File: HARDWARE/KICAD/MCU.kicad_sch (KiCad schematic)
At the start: 30 parts, among them U4 STM32F411RET6, Y1 12MHz 18pF, Y2 32.768kHz 12.5pF

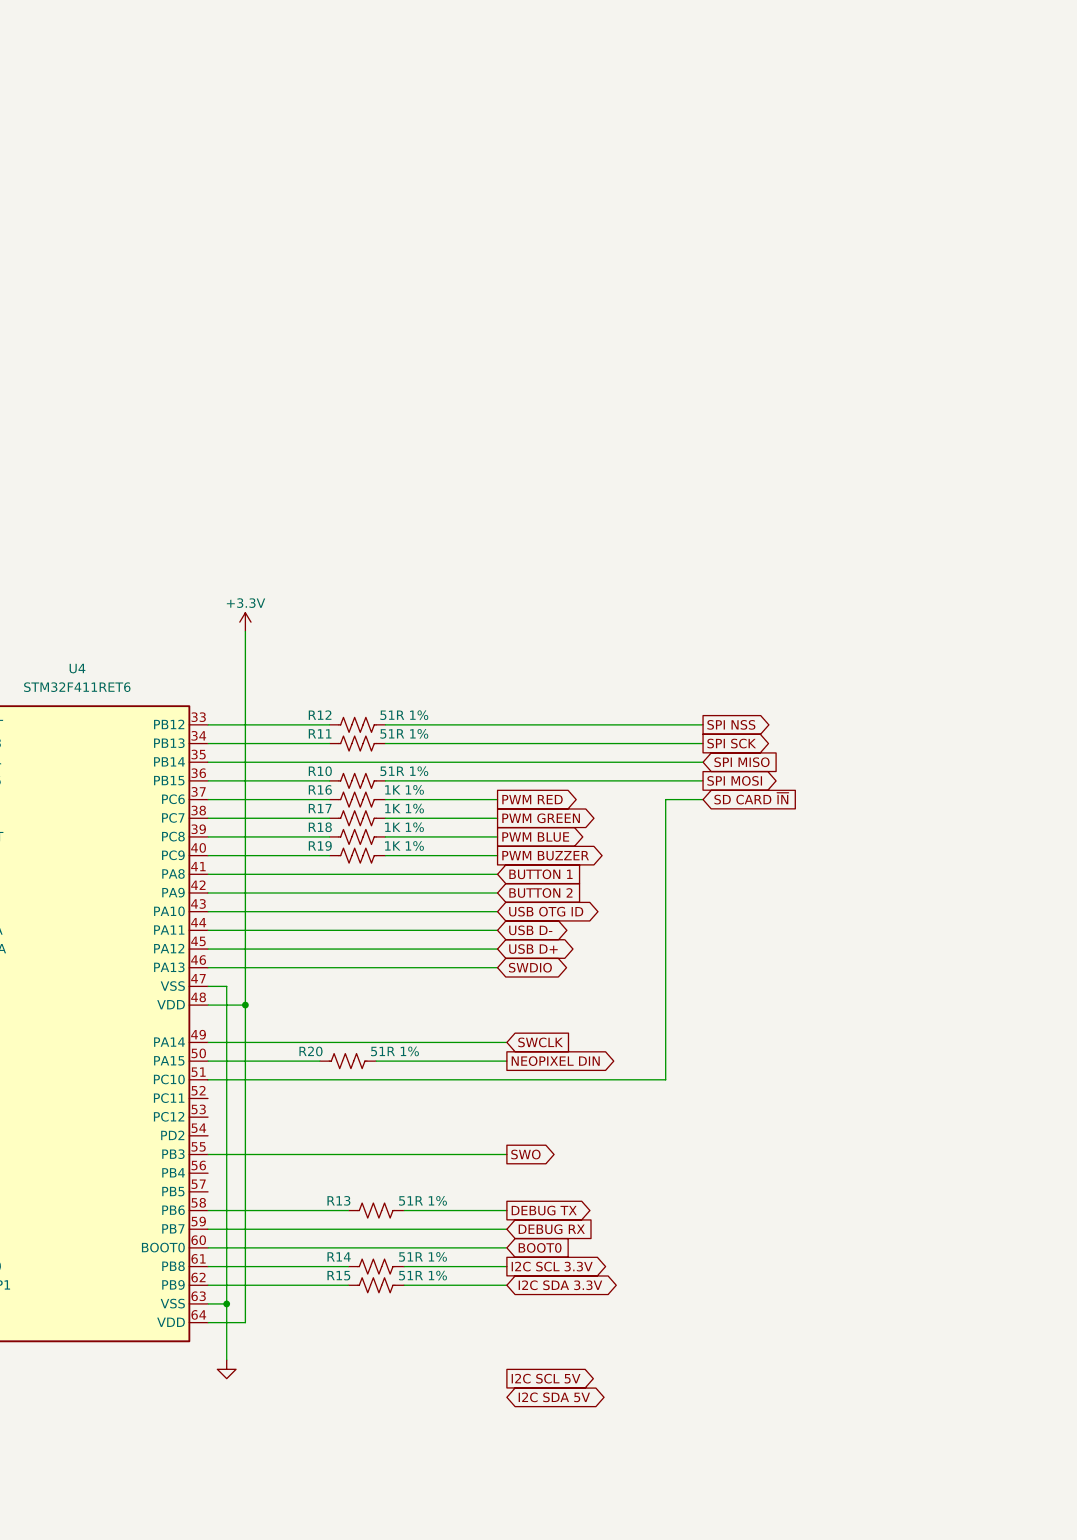
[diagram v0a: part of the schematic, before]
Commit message: Fixed MCU pins on schematic and routed I2C voltage translator.
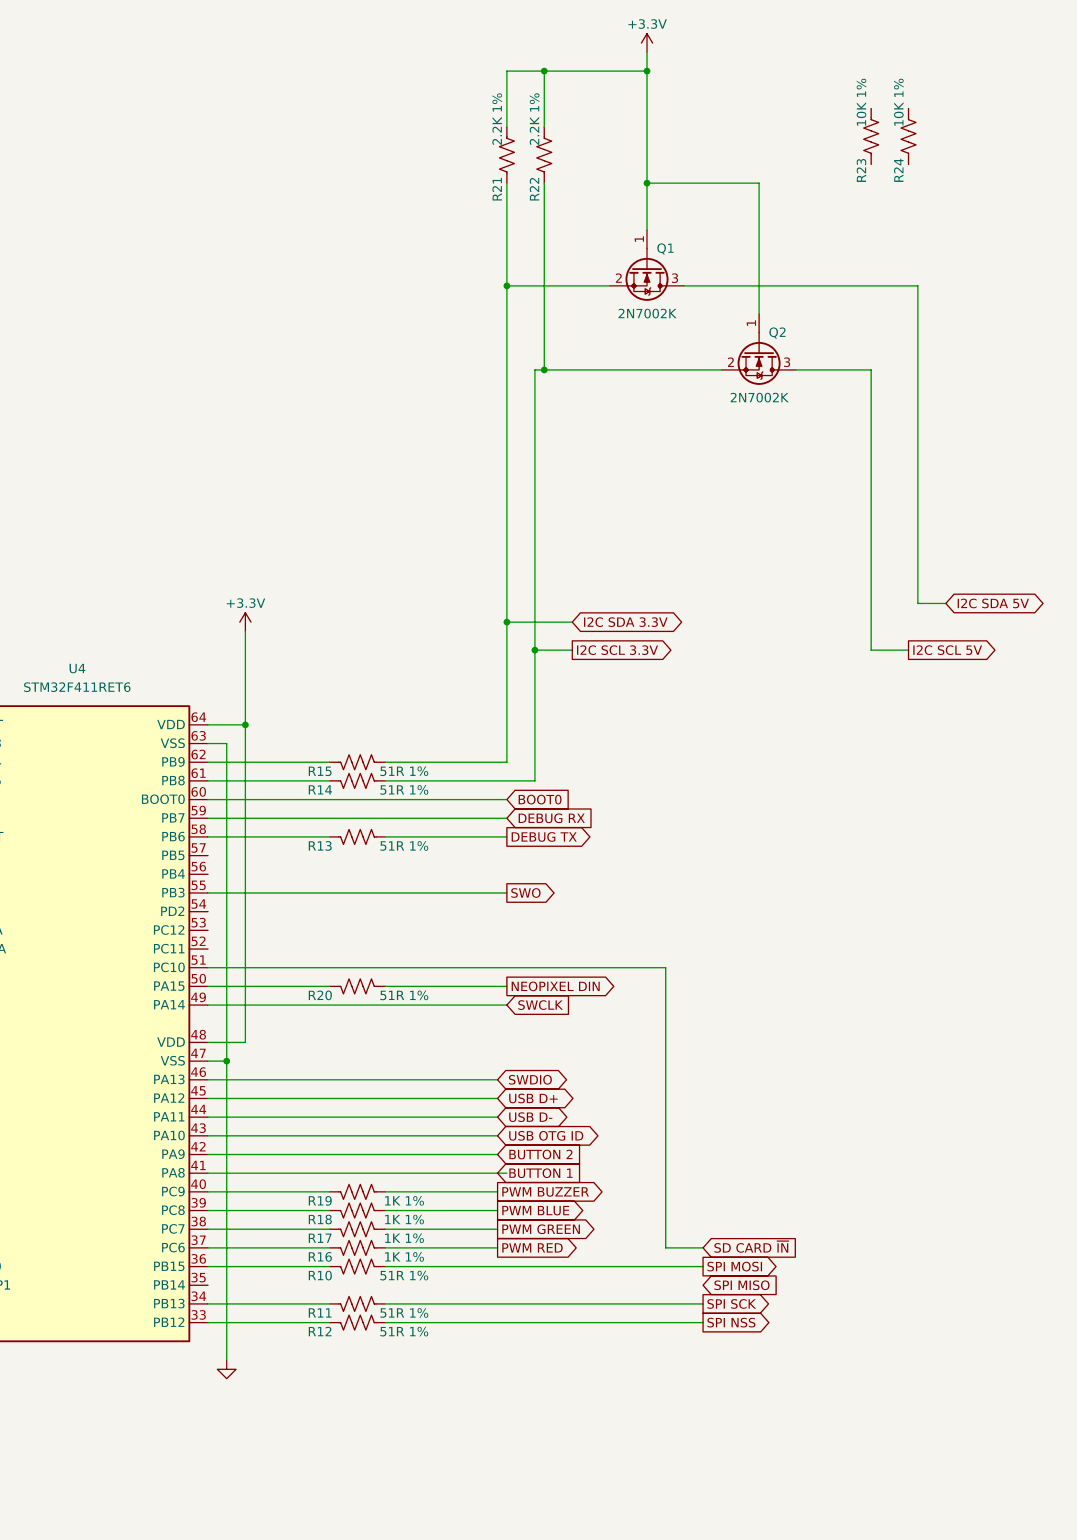
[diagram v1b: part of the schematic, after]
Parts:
- added Q1, Q2: 2N7002K, EMBARCADOS - CURSO PCB:SOT-23, symbol EMBARCADOS - CURSO PCB:TRANSISTOR 2N7002K-7
- added R21, R22: 2.2K 1%, EMBARCADOS - CURSO PCB:R_0603_1608Metric, symbol EMBARCADOS - CURSO PCB:RES 0603 2.2K 1% VISHAY CRCW06032K20FK
- added R23, R24: 10K 1%, EMBARCADOS - CURSO PCB:R_0603_1608Metric, symbol EMBARCADOS - CURSO PCB:RES 0603 10K 1% VISHAY CRCW060310K0FK
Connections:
- net +3.3V: now also Q1.1 (G), Q2.1 (G), R21.1, R22.1
- net I2C SCL 3.3V: now also Q2.2 (S), R22.2
- net I2C SCL 5V: now also Q2.3 (D)
- net I2C SDA 3.3V: now also Q1.2 (S), R21.2
- net I2C SDA 5V: now also Q1.3 (D)
- net SPI MISO: no longer U4.35 (PB14)
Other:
- moved on the sheet: R10, R11, R12, R13, R14, R15, R16, R17, R18, R19, R20

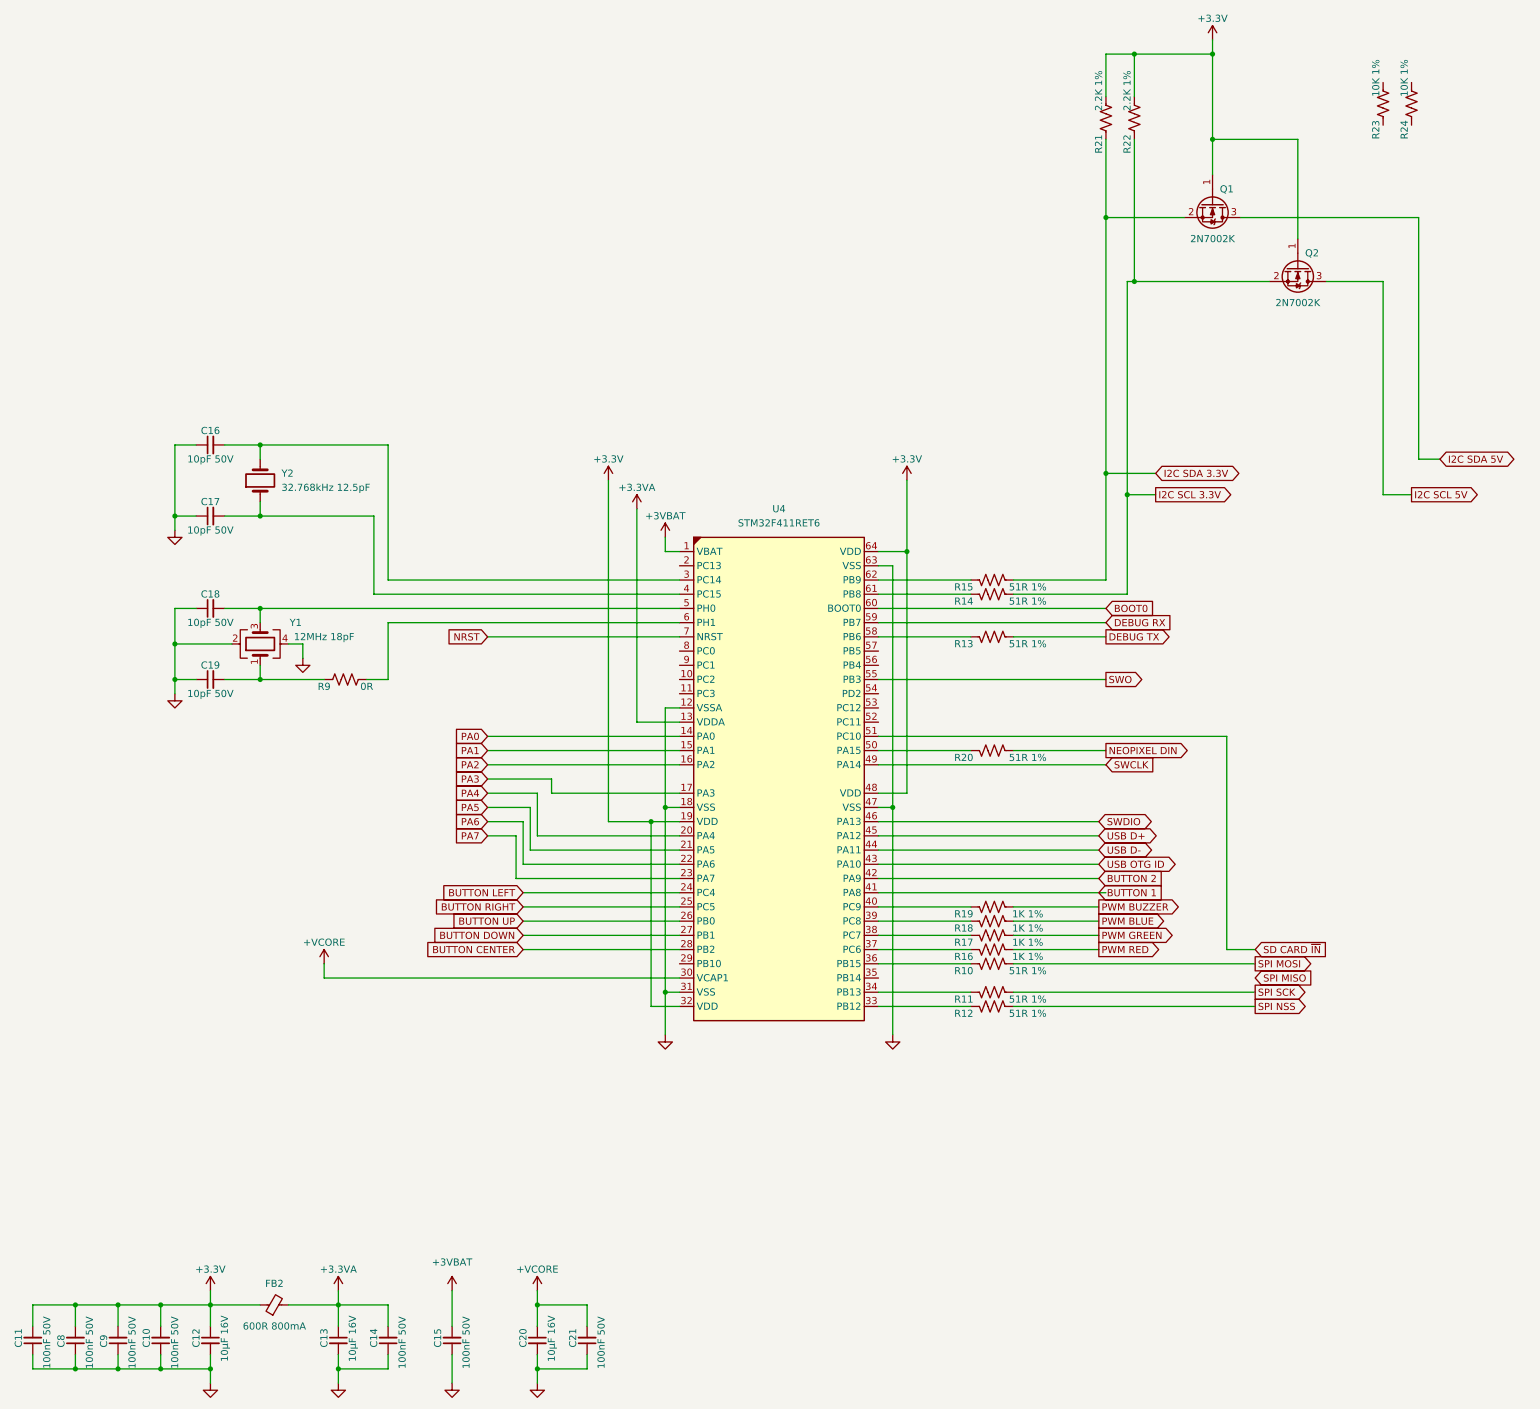
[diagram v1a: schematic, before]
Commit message: Refactoring.
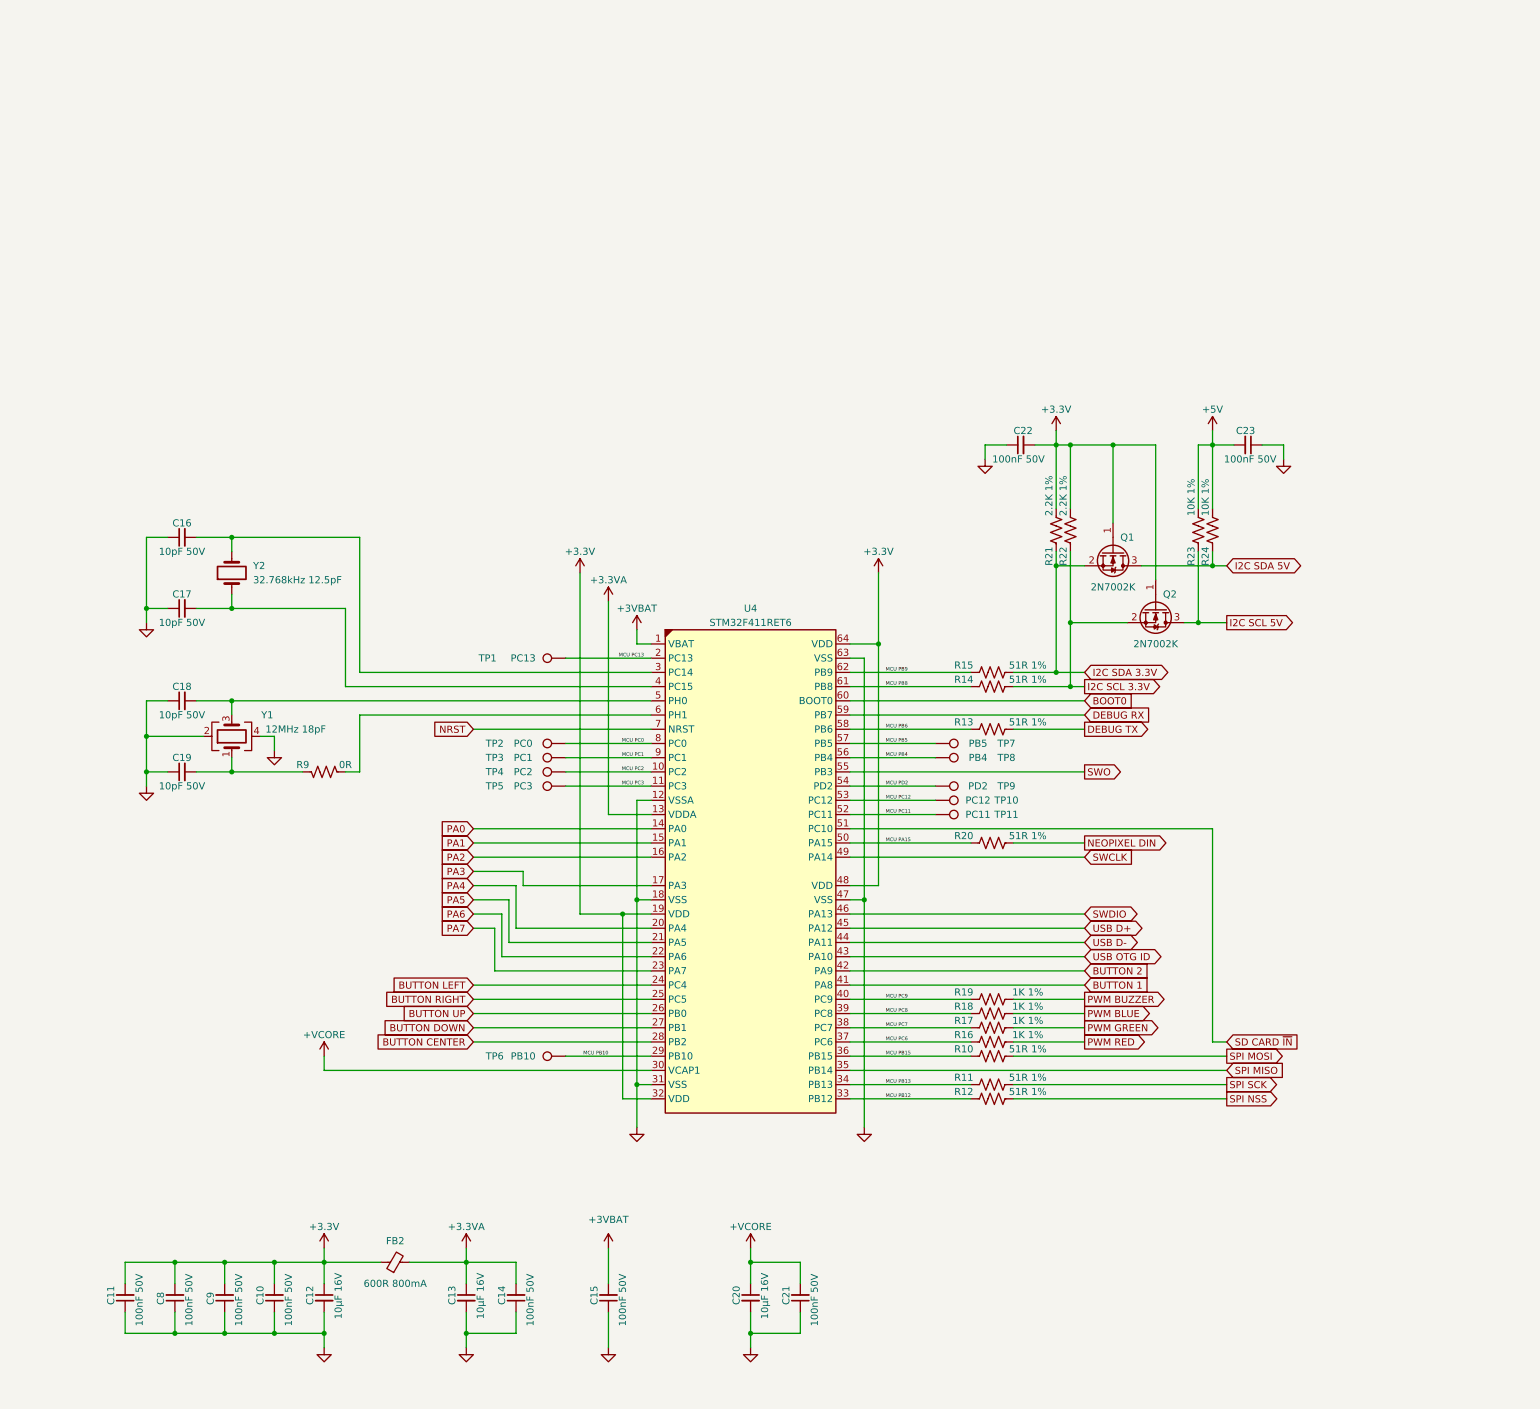
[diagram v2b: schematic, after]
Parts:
- added C22, C23: 100nF 50V, EMBARCADOS - CURSO PCB:C_0603_1608Metric, symbol EMBARCADOS - CURSO PCB:CAP 0603 100nF 50V AVX KGM15BR71H104K
- added TP1: PC13, symbol EMBARCADOS - CURSO PCB:AUX TEST POINT
- added TP10: PC12, symbol EMBARCADOS - CURSO PCB:AUX TEST POINT
- added TP11: PC11, symbol EMBARCADOS - CURSO PCB:AUX TEST POINT
- added TP2: PC0, symbol EMBARCADOS - CURSO PCB:AUX TEST POINT
- added TP3: PC1, symbol EMBARCADOS - CURSO PCB:AUX TEST POINT
- added TP4: PC2, symbol EMBARCADOS - CURSO PCB:AUX TEST POINT
- added TP5: PC3, symbol EMBARCADOS - CURSO PCB:AUX TEST POINT
- added TP6: PB10, symbol EMBARCADOS - CURSO PCB:AUX TEST POINT
- added TP7: PB5, symbol EMBARCADOS - CURSO PCB:AUX TEST POINT
- added TP8: PB4, symbol EMBARCADOS - CURSO PCB:AUX TEST POINT
- added TP9: PD2, symbol EMBARCADOS - CURSO PCB:AUX TEST POINT
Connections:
- net +3.3V: now also C22.2
- net GND: now also C22.1, C23.1
- net I2C SCL 5V: now also R23.2
- net I2C SDA 5V: now also R24.2
- net SPI MISO: now also U4.35 (PB14)
- net +5V: now reaches R23.1
- net +5V: now also R24.1, C23.2
- net MCU PB8: now reaches R14.1, U4.61 (PB8)
- net MCU PC2: now reaches U4.10 (PC2)
- net MCU PC2: now also TP4.1
- net MCU PC3: now reaches U4.11 (PC3)
- net MCU PC3: now also TP5.1
- net MCU PC13: now reaches U4.2 (PC13)
- net MCU PC13: now also TP1.1
- net MCU PB10: now reaches U4.29 (PB10)
- net MCU PB10: now also TP6.1
- net MCU PB12: now reaches R12.1, U4.33 (PB12)
- net MCU PB13: now reaches R11.1, U4.34 (PB13)
- net MCU PB15: now reaches R10.1, U4.36 (PB15)
- net MCU PC6: now reaches R16.1, U4.37 (PC6)
- net MCU PC7: now reaches R17.1, U4.38 (PC7)
- net MCU PC8: now reaches R18.1, U4.39 (PC8)
- net MCU PC9: now reaches R19.1, U4.40 (PC9)
- net MCU PA15: now reaches R20.1, U4.50 (PA15)
- net MCU PC11: now reaches U4.52 (PC11)
- net MCU PC11: now also TP11.1
- net MCU PC12: now reaches U4.53 (PC12)
- net MCU PC12: now also TP10.1
- net MCU PD2: now reaches U4.54 (PD2)
- net MCU PD2: now also TP9.1
- net MCU PB4: now reaches U4.56 (PB4)
- net MCU PB4: now also TP8.1
- net MCU PB5: now reaches U4.57 (PB5)
- net MCU PB5: now also TP7.1
- net MCU PB6: now reaches R13.1, U4.58 (PB6)
- net MCU PB9: now reaches R15.1, U4.62 (PB9)
- net MCU PC0: now reaches U4.8 (PC0)
- net MCU PC0: now also TP2.1
- net MCU PC1: now reaches U4.9 (PC1)
- net MCU PC1: now also TP3.1
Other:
- moved on the sheet: C10, C11, C12, C13, C14, C15, C16, C17, C18, C19, C20, C21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
